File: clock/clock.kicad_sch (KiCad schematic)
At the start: 43 parts, among them J1 Conn_01x06, J2 Power_inlet_vertical, J3 Conn_02x03_Odd_Even, J4 Conn_01x05, J5 Conn_01x05, SW1 Omron_B3F_SPST, SW2 Omron_B3F_SPST, SW3 Omron_B3F_SPST, SW4 Omron_B3F_SPST, U1 ATmega328-PU, U2 L7805, U3 MAX7219, U4 DS1307_DIP-8, Y1 Crystal_16MHz, Y2 Crystal_32768Hz

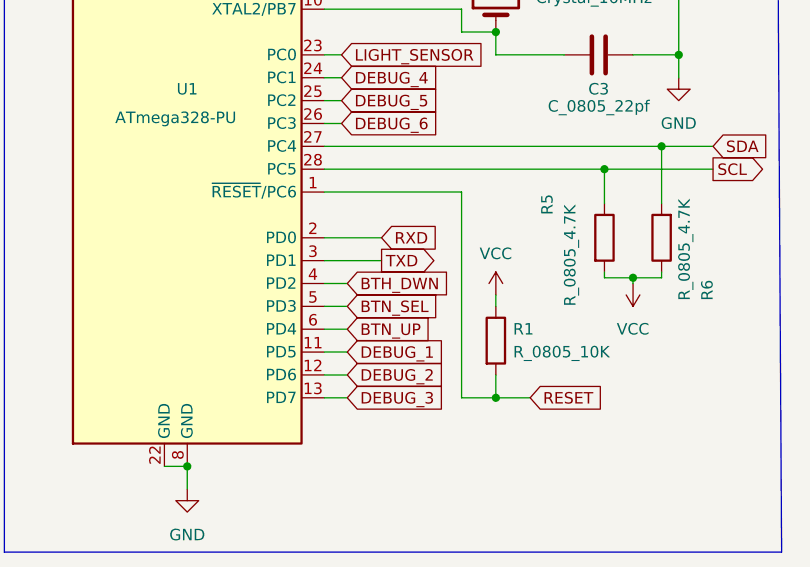
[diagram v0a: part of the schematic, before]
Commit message: pretty close to done
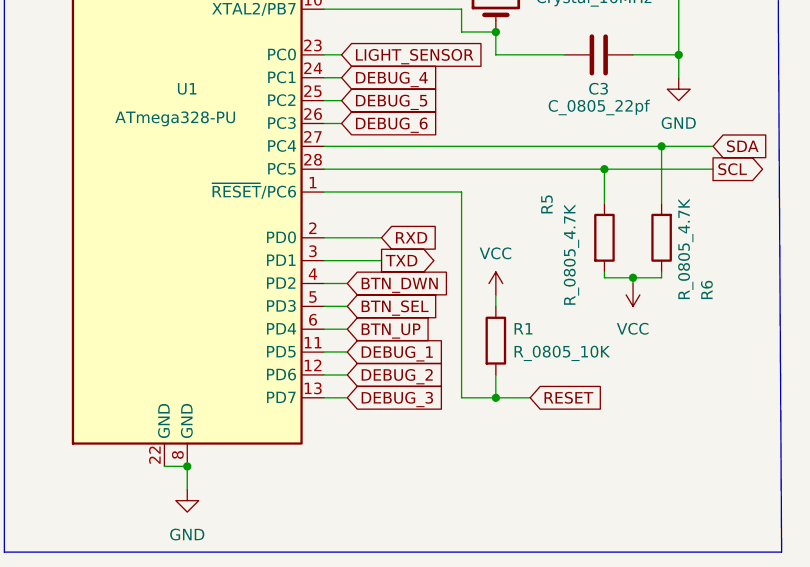
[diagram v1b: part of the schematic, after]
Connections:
- net BTH_DWN is gone; now on net BTN_DWN: U1.4 (PD2)
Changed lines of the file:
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@@
     )
   )
-  (global_label "BTH_DWN" (shape input) (at 54.61 97.79 0) (fields_autoplaced)
+  (global_label "BTN_DWN" (shape input) (at 54.61 97.79 0) (fields_autoplaced)
     (effects (font (size 1.27 1.27)) (justify left))
     (property "Intersheet References" "${INTERSHEET_REFS}" (id 0) (at 65.6107 97.7106 0)
